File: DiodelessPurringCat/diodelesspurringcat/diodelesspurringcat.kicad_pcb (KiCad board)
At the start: 2 copper layers, 114 x 92.4 mm, 21 parts, among them J1 ScreenL, U1 ProMicro-kbd

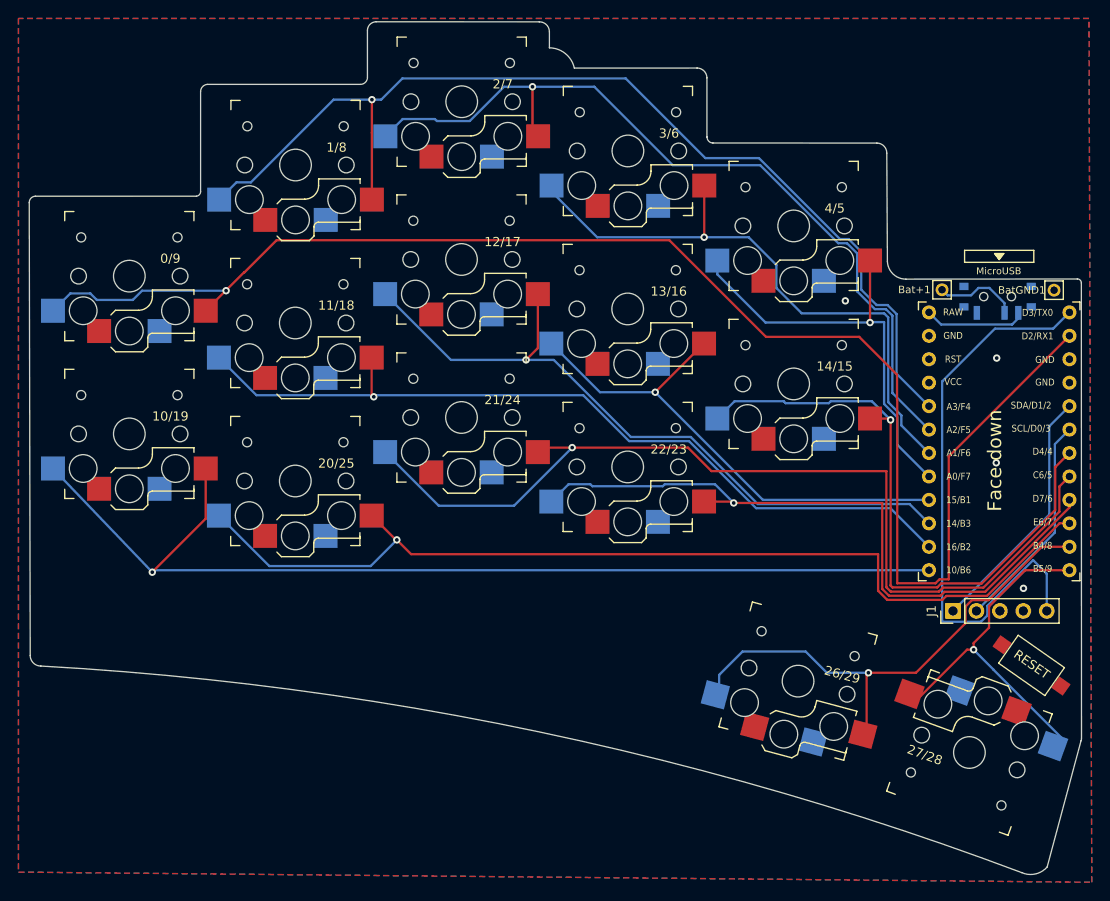
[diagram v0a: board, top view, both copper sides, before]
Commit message: trying to make a reversible nice view
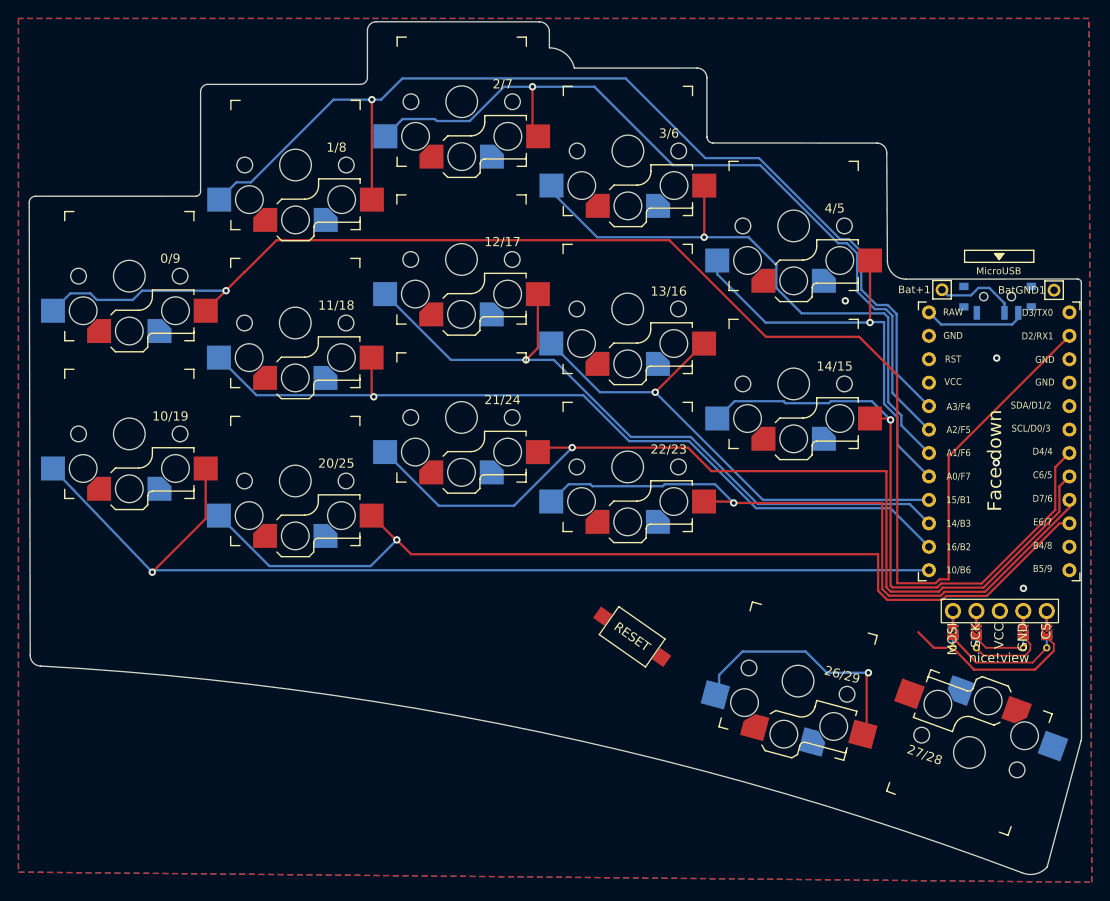
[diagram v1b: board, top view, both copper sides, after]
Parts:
- 0/9, 1/8, 10/19, 11/18, 12/17, 13/16, 14/15, 2/7, 20/25, 21/24, 22/23, 26/29, 27/28, 3/6, 4/5: footprint keyswitches:Kailh_socket_PG1350_reversible -> chelming-kbd:choc_v1_hotswap_reversible_no_extras
- J1: value ScreenL -> nice!view; footprint Connector_PinHeader_2.54mm:PinHeader_1x05_P2.54mm_Vertical -> chelming-kbd:nice-view_reversible
- moved RSW1 43.4 mm to (199.0, 85.0)
- moved J1 17.3 mm to (238.8, 65.7), turned to 0 degrees
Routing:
- net CS: track 62.3 -> 0.00 mm
- net s27: track 38.8 -> 0.00 mm, vias 1 -> 0
- net s26: track 54.7 -> 26.2 mm
- net MOSI: track 27.4 -> 0.00 mm
- net SCK: track 23.8 -> 0.00 mm
- net (no net): track 0.00 -> 3.74 mm
